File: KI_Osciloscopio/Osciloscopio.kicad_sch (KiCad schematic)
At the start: 40 parts, among them J1 Barrel Jack, U1 MCP6004, U2 74HC4051, U3 LM7805, U4 LM1117-3.3

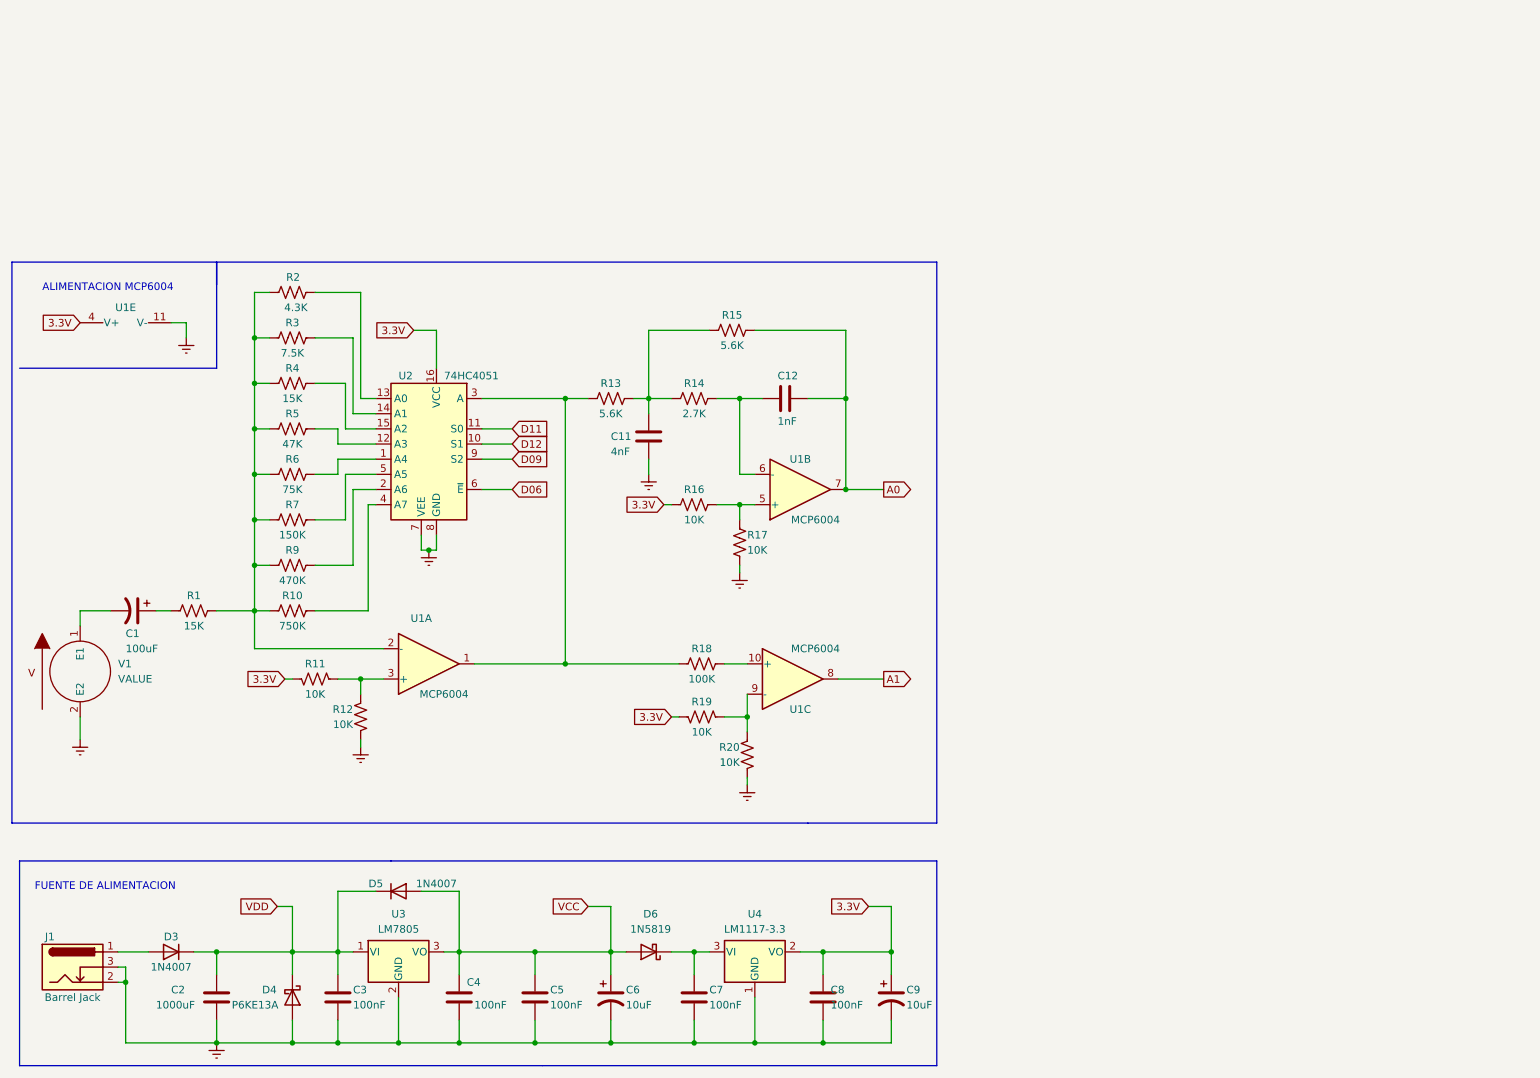
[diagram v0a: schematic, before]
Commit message: Esquematico terminado
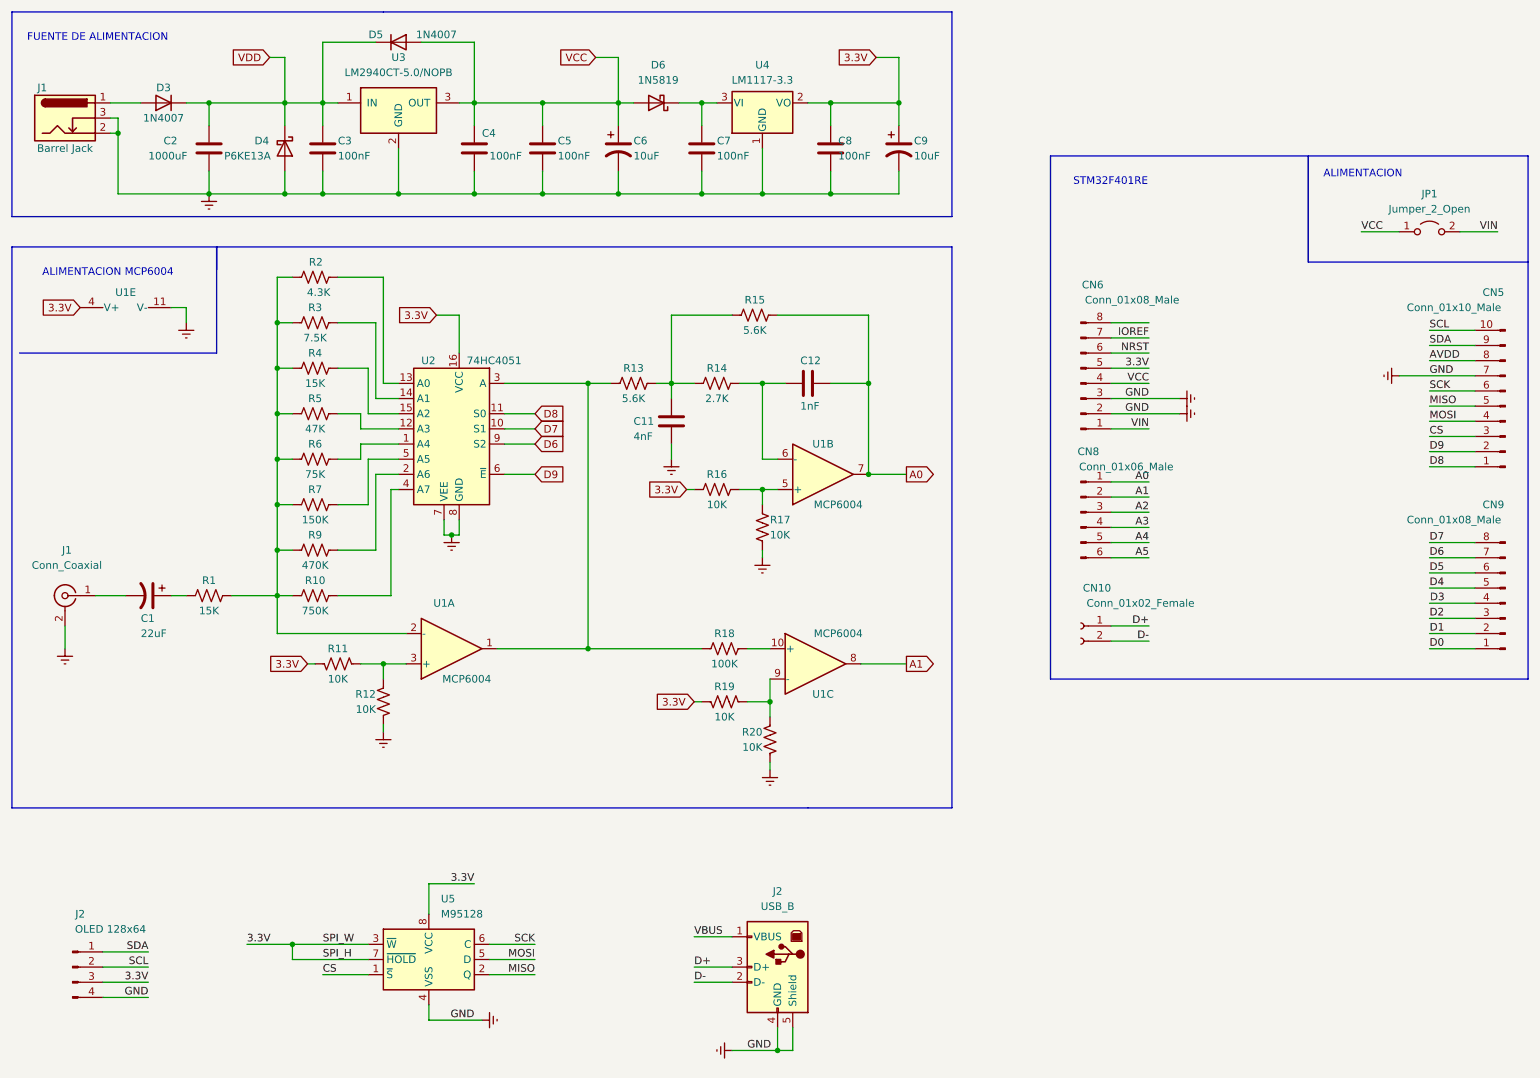
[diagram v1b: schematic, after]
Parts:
- removed U3: LM7805, Package_TO_SOT_THT:TO-220-3_Vertical, symbol Regulator_Linear:LM7805_TO220
- removed V1: VALUE, symbol pspice:VSOURCE
- added CN10: Conn_01x02_Female, symbol Connector:Conn_01x02_Female
- added CN5: Conn_01x10_Male, symbol Connector:Conn_01x10_Male
- added CN6, CN9: Conn_01x08_Male, symbol Connector:Conn_01x08_Male
- added CN8: Conn_01x06_Male, symbol Connector:Conn_01x06_Male
- added J1: Conn_Coaxial, symbol Connector:Conn_Coaxial
- added J2: USB_B, symbol Connector:USB_B
- added J2: OLED 128x64, symbol Connector:Conn_01x04_Male
- added JP1: Jumper_2_Open, symbol Jumper:Jumper_2_Open
- added U3: LM2940CT-5.0/NOPB, TO_SOT_Packages_THT:TO-220_Vertical, symbol AOI-LM2940CT:LM2940CT-5.0/NOPB
- added U5: M95128, Package_SO:SOIC-8_3.9x4.9mm_P1.27mm, symbol Memory_EEPROM:M95256-WMN6P
- C1: value 100uF -> 22uF
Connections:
- net 3.3V: now also CN6.5 (Pin_5), J2.3 (Pin_3), U5.3 (~{W}), U5.7 (~{HOLD}), U5.8 (VCC)
- net A0: now also CN8.1 (Pin_1)
- net A1: now also CN8.2 (Pin_2)
- net Earth: now also U3.2 (GND)
- net GNDREF: now also CN5.7 (Pin_7), CN6.2 (Pin_2), CN6.3 (Pin_3), J1.2 (Ext), J2.4 (GND), J2.4 (Pin_4), J2.5 (Shield), U5.4 (VSS)
- net VCC: now also CN6.4 (Pin_4), JP1.1 (A), U3.3 (OUT)
- net VDD: now also U3.1 (IN)
- net at C1.2: now also J1.1 (In)
- net D06 renamed D9
- net D9: now also CN5.2 (Pin_2)
- net D09 renamed D6
- net D6: now also CN9.7 (Pin_7)
- net D11 renamed D8
- net D8: now also CN5.1 (Pin_1)
- net D12 renamed D7
- net D7: now also CN9.8 (Pin_8)
- new net A2: CN8.3 (Pin_3)
- new net A3: CN8.4 (Pin_4)
- new net A4: CN8.5 (Pin_5)
- new net A5: CN8.6 (Pin_6)
- new net AVDD: CN5.8 (Pin_8)
- new net CS: CN5.3 (Pin_3), U5.1 (~{S})
- new net D+: CN10.1 (Pin_1), J2.3 (D+)
- new net D-: CN10.2 (Pin_2), J2.2 (D-)
- new net D0: CN9.1 (Pin_1)
- new net D1: CN9.2 (Pin_2)
- new net D2: CN9.3 (Pin_3)
- new net D3: CN9.4 (Pin_4)
- new net D4: CN9.5 (Pin_5)
- new net D5: CN9.6 (Pin_6)
- new net IOREF: CN6.7 (Pin_7)
- new net MISO: CN5.5 (Pin_5), U5.2 (Q)
- new net MOSI: CN5.4 (Pin_4), U5.5 (D)
- new net NRST: CN6.6 (Pin_6)
- new net SCK: CN5.6 (Pin_6), U5.6 (C)
- new net SCL: CN5.10 (Pin_10), J2.2 (Pin_2)
- new net SDA: CN5.9 (Pin_9), J2.1 (Pin_1)
- new net VBUS: J2.1 (VBUS)
- new net VIN: CN6.1 (Pin_1), JP1.2 (B)
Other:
- note added: "ALIMENTACION"
- note added: "STM32F401RE"
- moved on the sheet: C1, C11, C12, C2, C3, C4, C5, C6, C7, C8, C9, D3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
